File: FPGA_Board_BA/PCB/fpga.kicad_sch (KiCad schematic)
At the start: 5 parts, among them J9 Box_Header_26pin, U2 Zynq7020

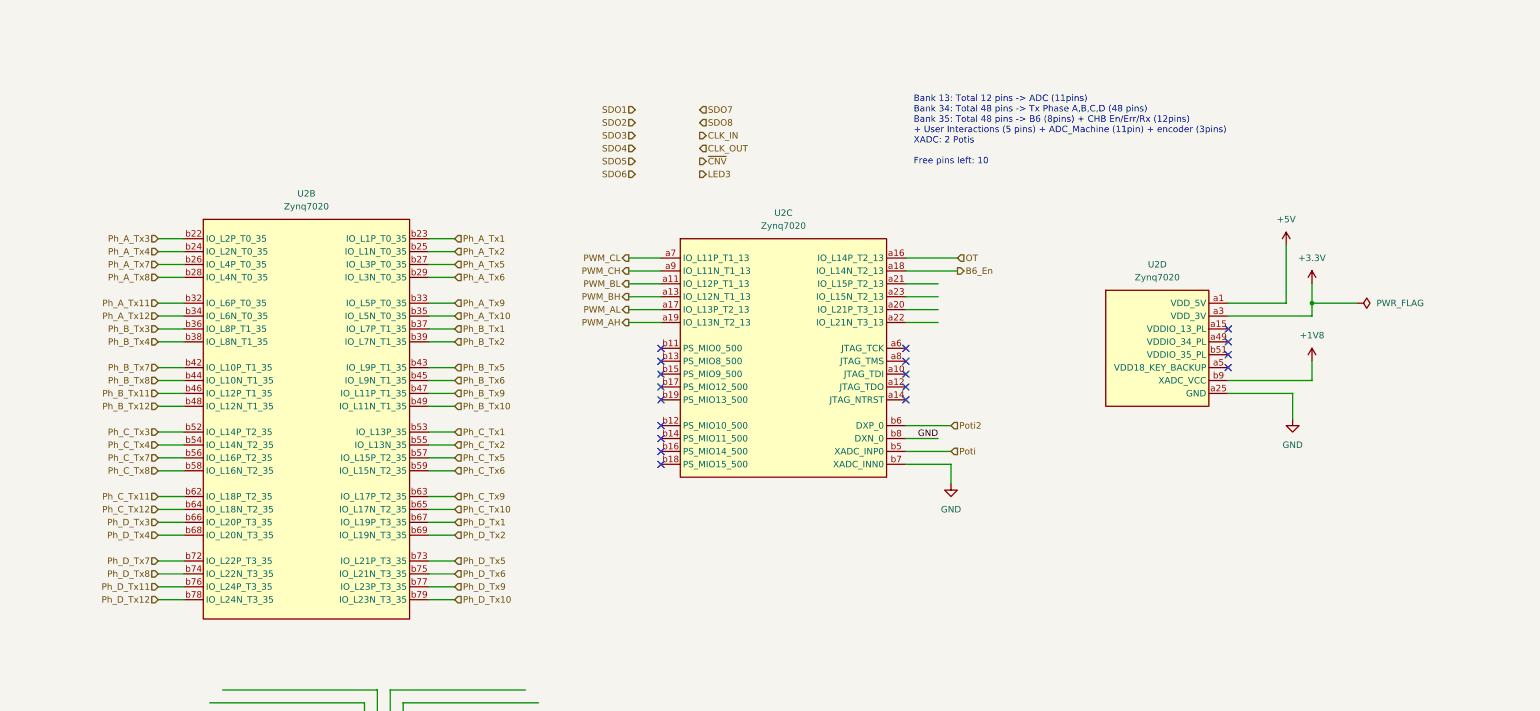
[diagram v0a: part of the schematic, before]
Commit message: some minimal changes on the PCB on the right side
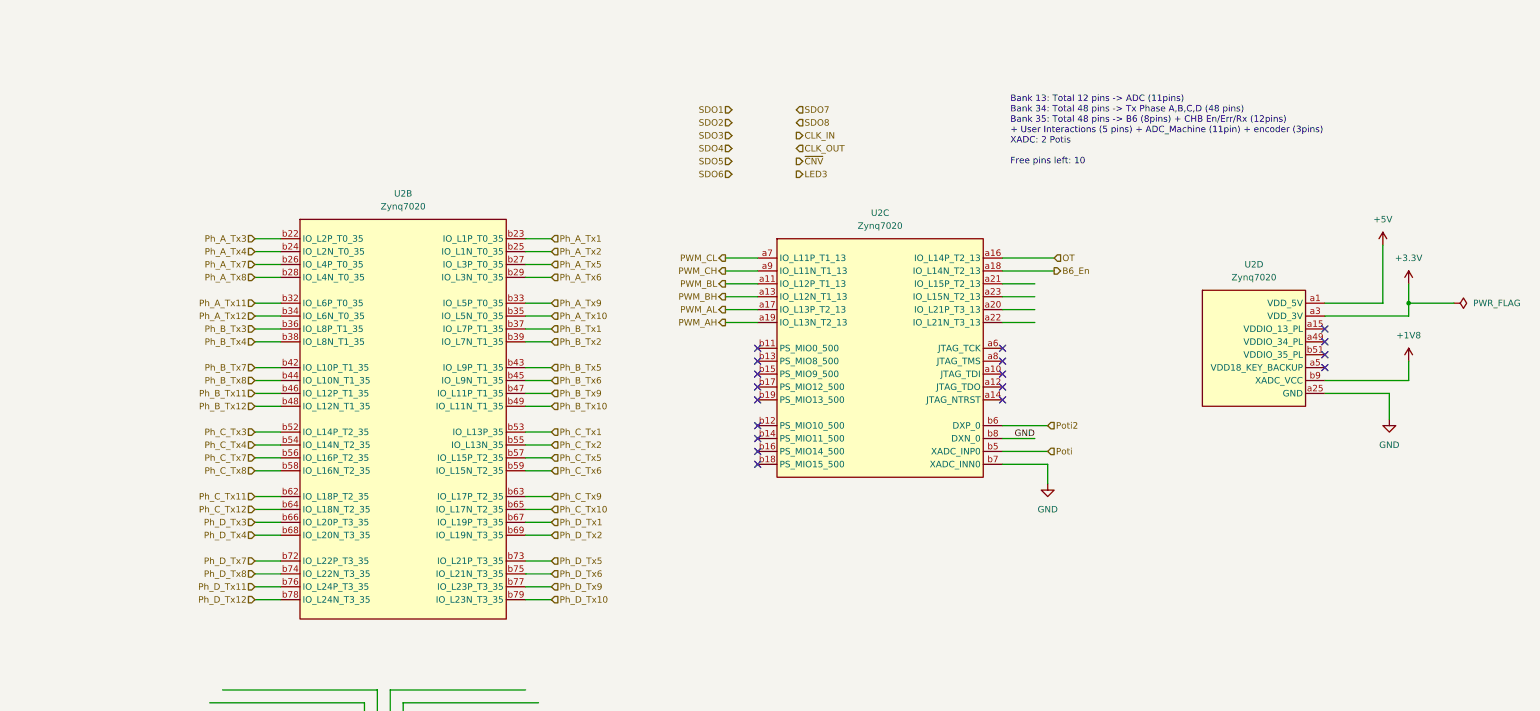
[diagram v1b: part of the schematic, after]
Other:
- moved on the sheet: U2B, U2C, U2D
